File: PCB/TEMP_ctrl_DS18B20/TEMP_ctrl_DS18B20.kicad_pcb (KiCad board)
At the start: 2 copper layers, 61.8 x 76 mm, 45 parts, among them J1 Heater2, J10 Heater3, J11 Heater2, J12 Heater4, J2 Heater4, J5 Conn_01x01_Pin, J6 Conn_01x01_Pin, J7 LCD, J9 Heater1, Q1 IRLZ44N, Q2 IRLZ44N, Q3 IRLZ44N, Q4 IRLZ44N, Q5 IRLZ44N, Q6 IRLZ44N, U1 STM32G431CBTx, U3 AP2112K-3.3, Y2 32KHz, Y3 ECS-160-12-33-AGN-TR3

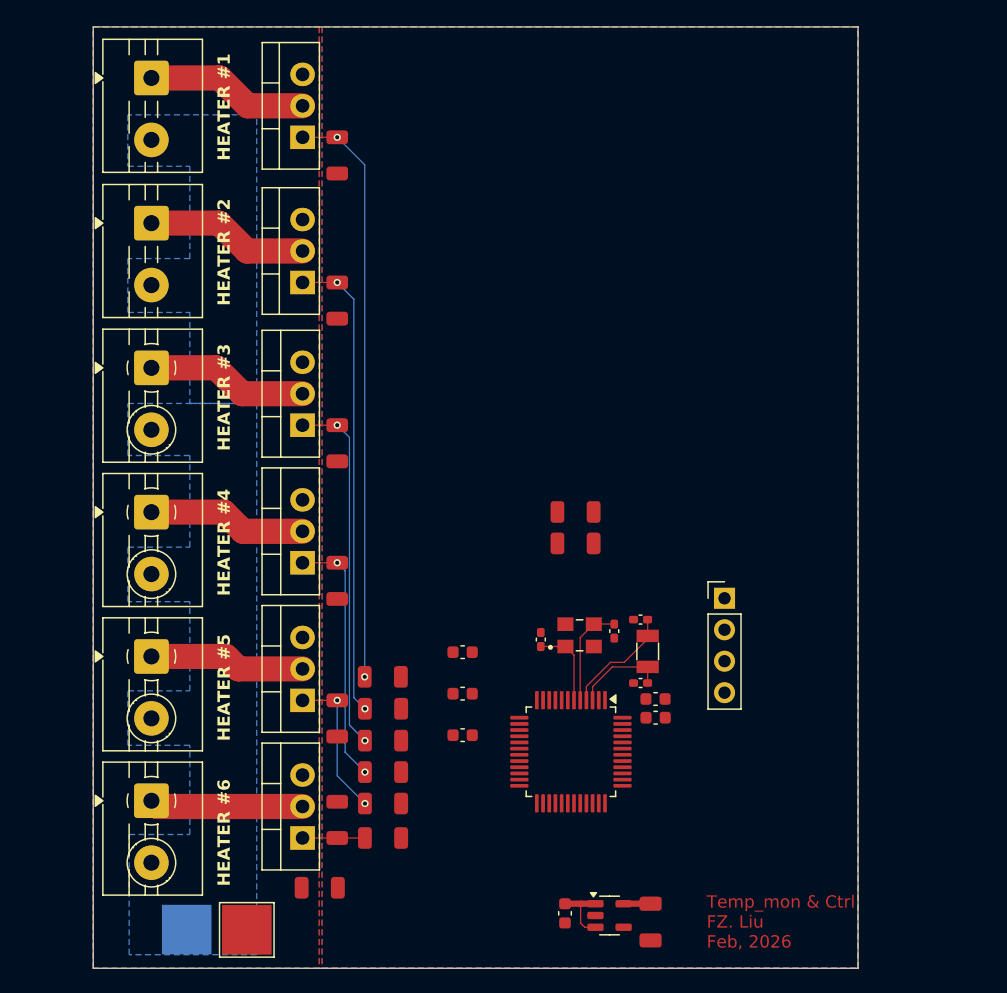
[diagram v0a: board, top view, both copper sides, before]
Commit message: PC: working on the DS18B20 PCB design
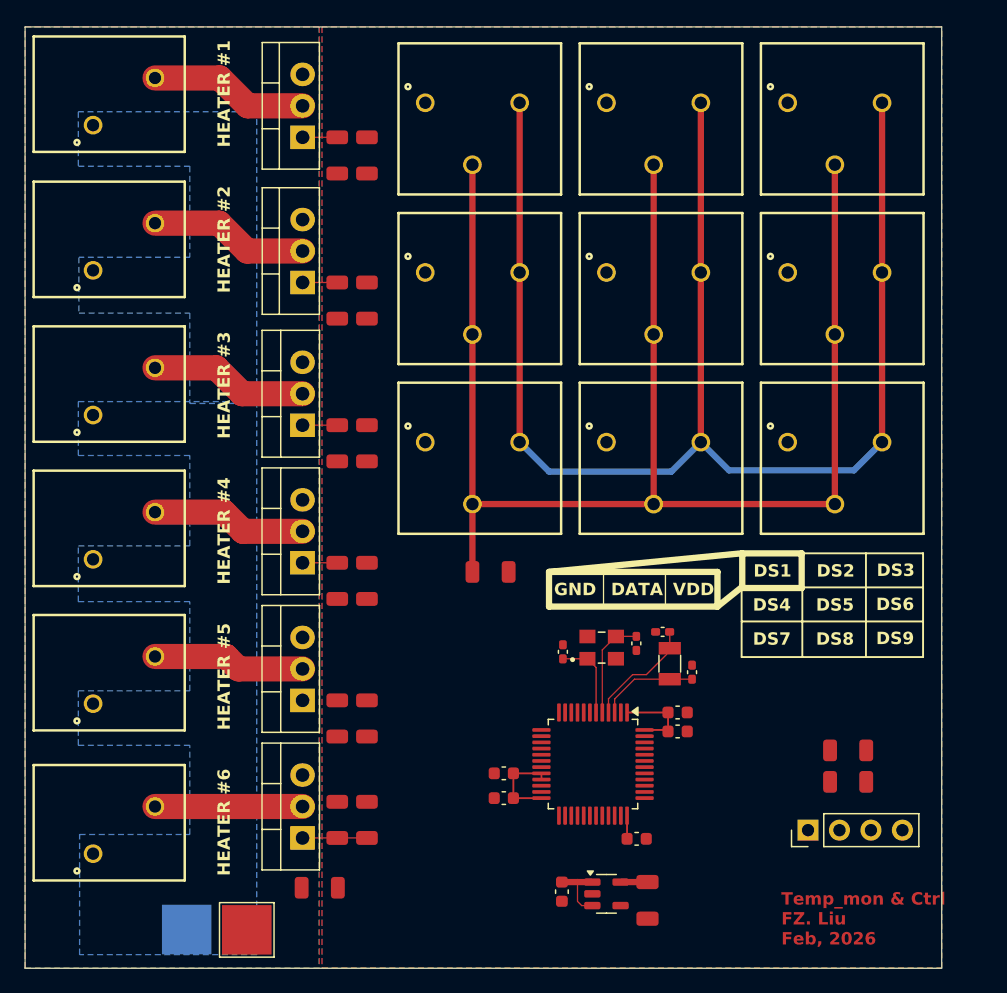
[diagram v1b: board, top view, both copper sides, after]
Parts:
- added J13: 691412320003, Mylib:691412320003, F.Cu at (155.2, 102.0)
- added J14: 691412320003, Mylib:691412320003, F.Cu at (155.2, 88.3)
- added J15: 691412320003, Mylib:691412320003, F.Cu at (155.2, 74.6)
- added J16: 691412320003, Mylib:691412320003, F.Cu at (140.6, 102.0)
- added J17: 691412320003, Mylib:691412320003, F.Cu at (140.6, 88.3)
- added J18: 691412320003, Mylib:691412320003, F.Cu at (140.6, 74.6)
- added J3: 691412320002, Mylib:691412320002, F.Cu at (112.5, 95.4)
- added J4: 691412320002, Mylib:691412320002, F.Cu at (112.5, 107.1)
- added J8: 691412320002, Mylib:691412320002, F.Cu at (112.5, 72.0)
- added R1: 4.7kΩ, PCM_JLCPCB:R_1206, F.Cu at (142.1, 110.0)
- J1: value Heater2 -> 691412320002; footprint TerminalBlock:TerminalBlock_MaiXu_MX126-5.0-02P_1x02_P5.00mm -> Mylib:691412320002
- J10: value Heater3 -> 691412320003; footprint TerminalBlock:TerminalBlock_MaiXu_MX126-5.0-02P_1x02_P5.00mm -> Mylib:691412320003
- J11: value Heater2 -> 691412320003; footprint TerminalBlock:TerminalBlock_MaiXu_MX126-5.0-02P_1x02_P5.00mm -> Mylib:691412320003
- J12: value Heater4 -> 691412320003; footprint TerminalBlock:TerminalBlock_MaiXu_MX126-5.0-02P_1x02_P5.00mm -> Mylib:691412320003
- J2: value Heater4 -> 691412320002; footprint TerminalBlock:TerminalBlock_MaiXu_MX126-5.0-02P_1x02_P5.00mm -> Mylib:691412320002
- J9: value Heater1 -> 691412320002; footprint TerminalBlock:TerminalBlock_MaiXu_MX126-5.0-02P_1x02_P5.00mm -> Mylib:691412320002
- moved J12 77.1 mm to (169.9, 74.6), turned to 180 degrees
- moved J11 57.7 mm to (169.9, 88.3), turned to 180 degrees
- moved J10 57.1 mm to (169.9, 102.0), turned to 180 degrees
- moved J2 49.1 mm to (112.5, 130.8)
- moved J1 48.7 mm to (112.5, 118.7)
- moved R2 42.1 mm to (132.1, 76.4), turned to 90 degrees
- moved R4 33.0 mm to (132.1, 88.1), turned to 90 degrees
- moved R27 29.2 mm to (170.9, 124.4)
- moved R28 29.2 mm to (170.9, 127.0)
- moved R19 24.0 mm to (132.1, 99.6), turned to 90 degrees
- moved J7 19.9 mm to (167.7, 130.8), turned to 90 degrees
- moved C3 18.3 mm to (153.9, 131.6)
- moved R20 15.5 mm to (132.1, 110.7), turned to 90 degrees
- moved C2 12.2 mm to (143.2, 128.3), turned to 180 degrees
- moved J9 10.0 mm to (112.5, 83.7)
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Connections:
- C22 pad 2: GND -> GNDD
- C23 pad 1: GND -> GNDD
- C24 pad 1: GND -> GNDD
- C26 pad 2: GND -> GNDD
- J1 pad 1: Net-(J1-Pin_1) -> +24V
- J1 pad 2: +24V -> Net-(Q4-D)
- J10 pad 1: Net-(J10-Pin_1) -> GNDD
- J10 pad 2: +24V -> DS_D
- J11 pad 1: Net-(J11-Pin_1) -> GNDD
- J11 pad 2: +24V -> DS_D
- J12 pad 1: Net-(J12-Pin_1) -> GNDD
- J12 pad 2: +24V -> DS_D
- J2 pad 1: Net-(J2-Pin_1) -> +24V
- J2 pad 2: +24V -> Net-(Q5-D)
- J9 pad 1: Net-(J9-Pin_1) -> +24V
- J9 pad 2: +24V -> Net-(Q6-D)
- Q1 pad 2: Net-(J11-Pin_1) -> Net-(Q1-D)
- Q2 pad 2: Net-(J9-Pin_1) -> Net-(Q2-D)
- Q3 pad 2: Net-(J1-Pin_1) -> Net-(Q3-D)
- Q4 pad 2: Net-(J10-Pin_1) -> Net-(Q4-D)
- Q5 pad 2: Net-(J12-Pin_1) -> Net-(Q5-D)
- Q6 pad 2: Net-(J2-Pin_1) -> Net-(Q6-D)
- Y3 pad 2: GND -> GNDD
- Y3 pad 4: GND -> GNDD
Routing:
- net DS_D: track 0.00 -> 116.9 mm
- net +3.3V: track 0.00 -> 115.3 mm
- net Net-(Q3-G): track 47.3 -> 2.79 mm, vias 2 -> 0
- net Net-(Q6-G): track 38.1 -> 2.79 mm, vias 2 -> 0
- net Net-(Q2-G): track 29.2 -> 2.80 mm, vias 2 -> 0
- net Net-(Q1-G): track 20.6 -> 2.80 mm, vias 2 -> 0
- net VAA: track 2.18 -> 17.9 mm
- net Net-(J2-Pin_1): track 13.1 -> 0.00 mm
- net Net-(J1-Pin_1): track 13.1 -> 0.00 mm
- net Net-(J9-Pin_1): track 13.1 -> 0.00 mm
- net Net-(Q6-D): track 0.00 -> 12.8 mm
- net Net-(Q3-D): track 0.00 -> 12.8 mm
- net Net-(J11-Pin_1): track 12.8 -> 0.00 mm
- net Net-(Q2-D): track 0.00 -> 12.8 mm
- net Net-(J10-Pin_1): track 12.6 -> 0.00 mm
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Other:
- board size 61.8 x 76 mm -> 74 x 76 mm
- board text added: "DATA"
- board text added: "DS1"
- board text added: "DS2"
- board text added: "DS3"
- board text added: "DS4"
- board text added: "DS5"
- board text added: "DS6"
- board text added: "DS7"
- board text added: "DS8"
- board text added: "DS9"
- board text added: "GND"
- board text added: "VDD"
